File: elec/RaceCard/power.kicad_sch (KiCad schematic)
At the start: 6 parts, among them Q1 DMP3125L-7, U1 TLV74033PDQNR

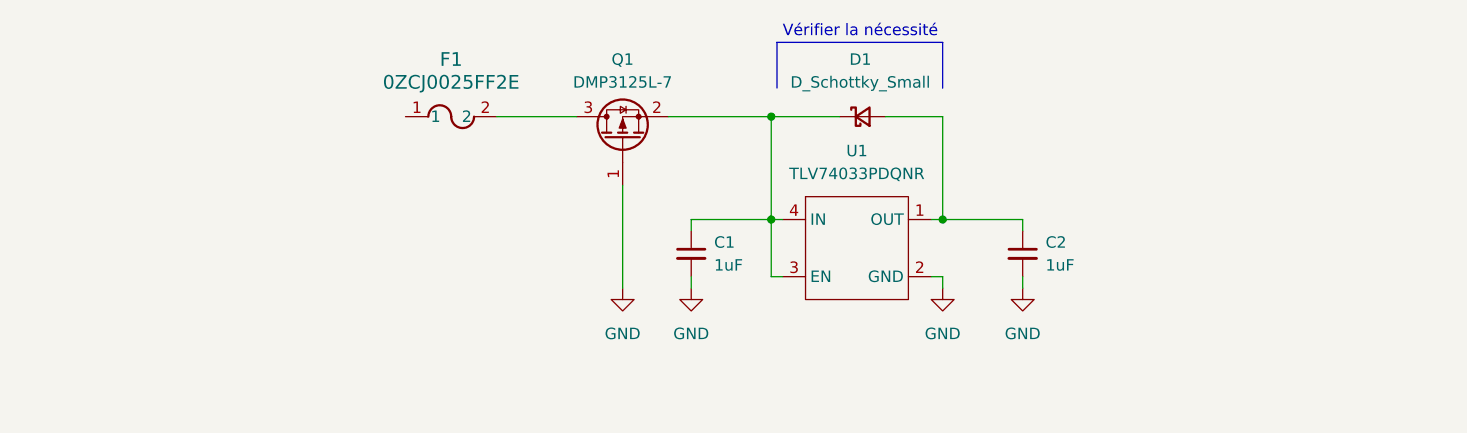
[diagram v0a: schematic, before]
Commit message: V1 du chargeur fini
Valider par qqn d'autre que Hugo
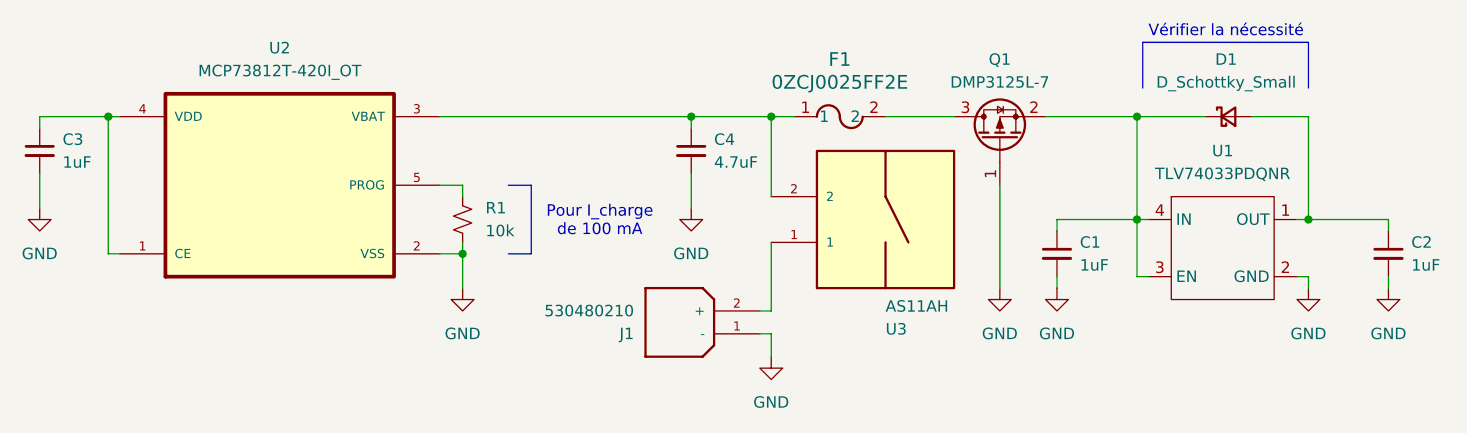
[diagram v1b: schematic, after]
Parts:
- added C3: 1uF, Capacitor_SMD:C_0603_1608Metric, symbol Device:C_Small
- added C4: 4.7uF, Capacitor_SMD:C_0603_1608Metric, symbol Device:C_Small
- added J1: 530480210, 530480210:MOLEX_530480210, symbol C3I_A25:530480210
- added R1: 10k, Resistor_SMD:R_0603_1608Metric, symbol Device:R_Small_US
- added U2: MCP73812T-420I_OT, MCP73812T-420I_OT:SOT95P280X145-5N, symbol C3I_A25:MCP73812T-420I_OT
- added U3: AS11AH, AS11AH:AS11AH, symbol C3I_A25:AS11AH
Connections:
- net GND: now also C3.2, C4.2, J1.1 (-), R1.2, U2.2 (VSS)
- net at F1.1: now also C4.1, U2.3 (VBAT), U3.2
- new net: R1.1, U2.5 (PROG)
- new net: J1.2 (+), U3.1
- new net: C3.1, U2.1 (CE), U2.4 (VDD)
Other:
- note added: "Pour I_charge de 100 mA"
- moved on the sheet: C1, C2, D1, F1, Q1, U1
